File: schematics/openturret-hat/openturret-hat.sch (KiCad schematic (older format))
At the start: 6 parts, among them J1 Raspberry_Pi_2_3, U0 L293D, U1 L293D, U2 AMS1117-5.0, U3 AMS1117-5.0

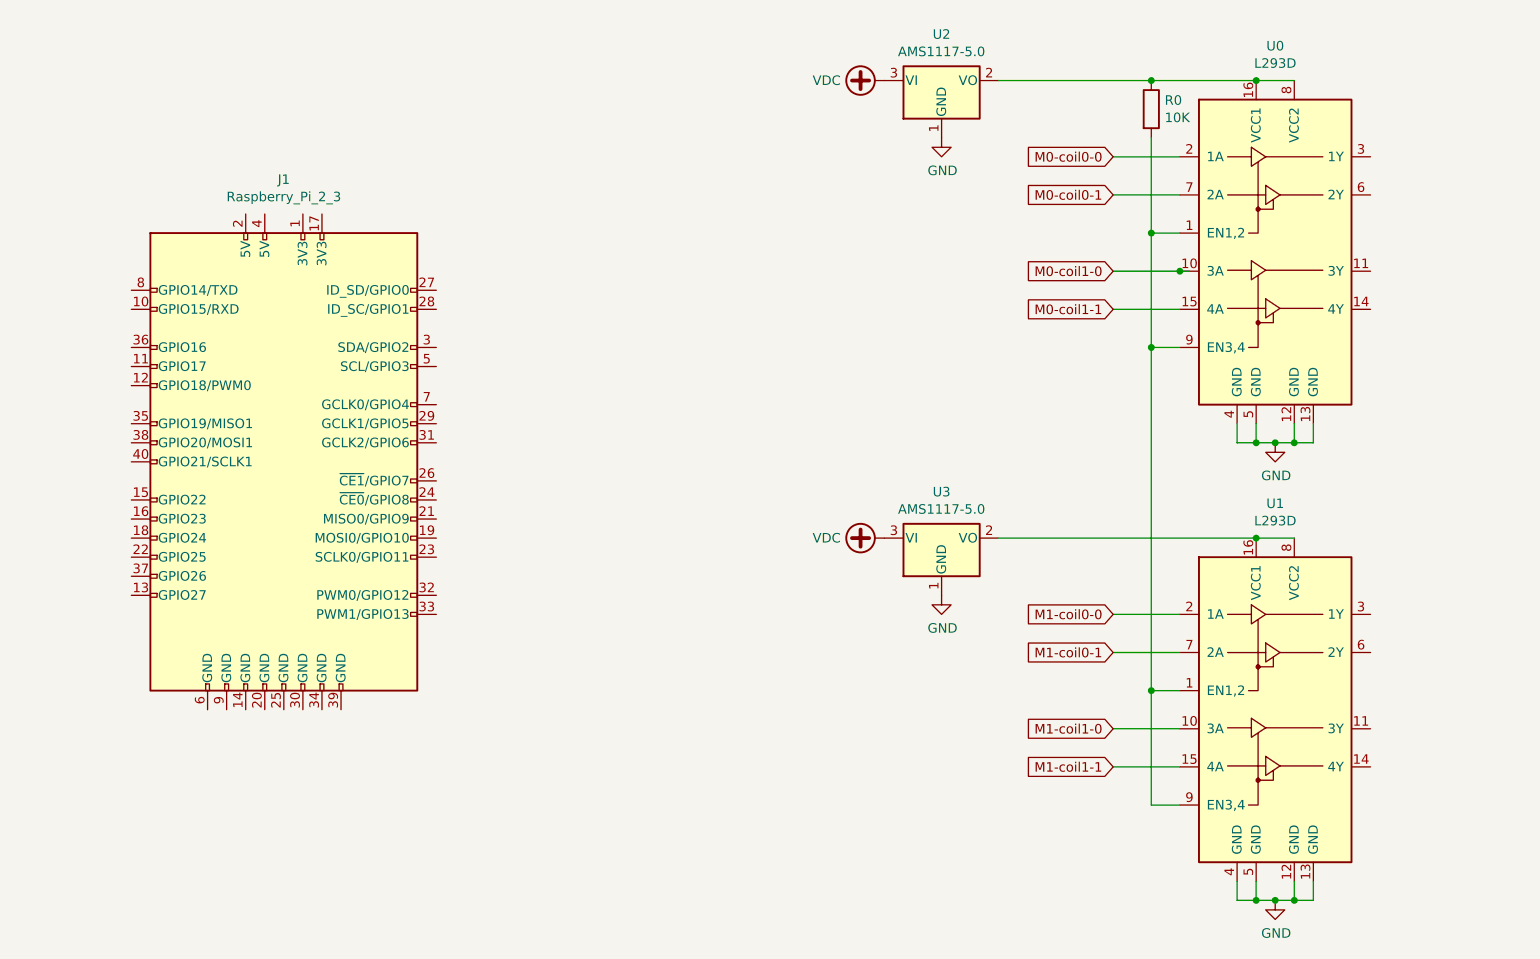
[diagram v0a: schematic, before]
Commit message: WIP on schematic and board layout
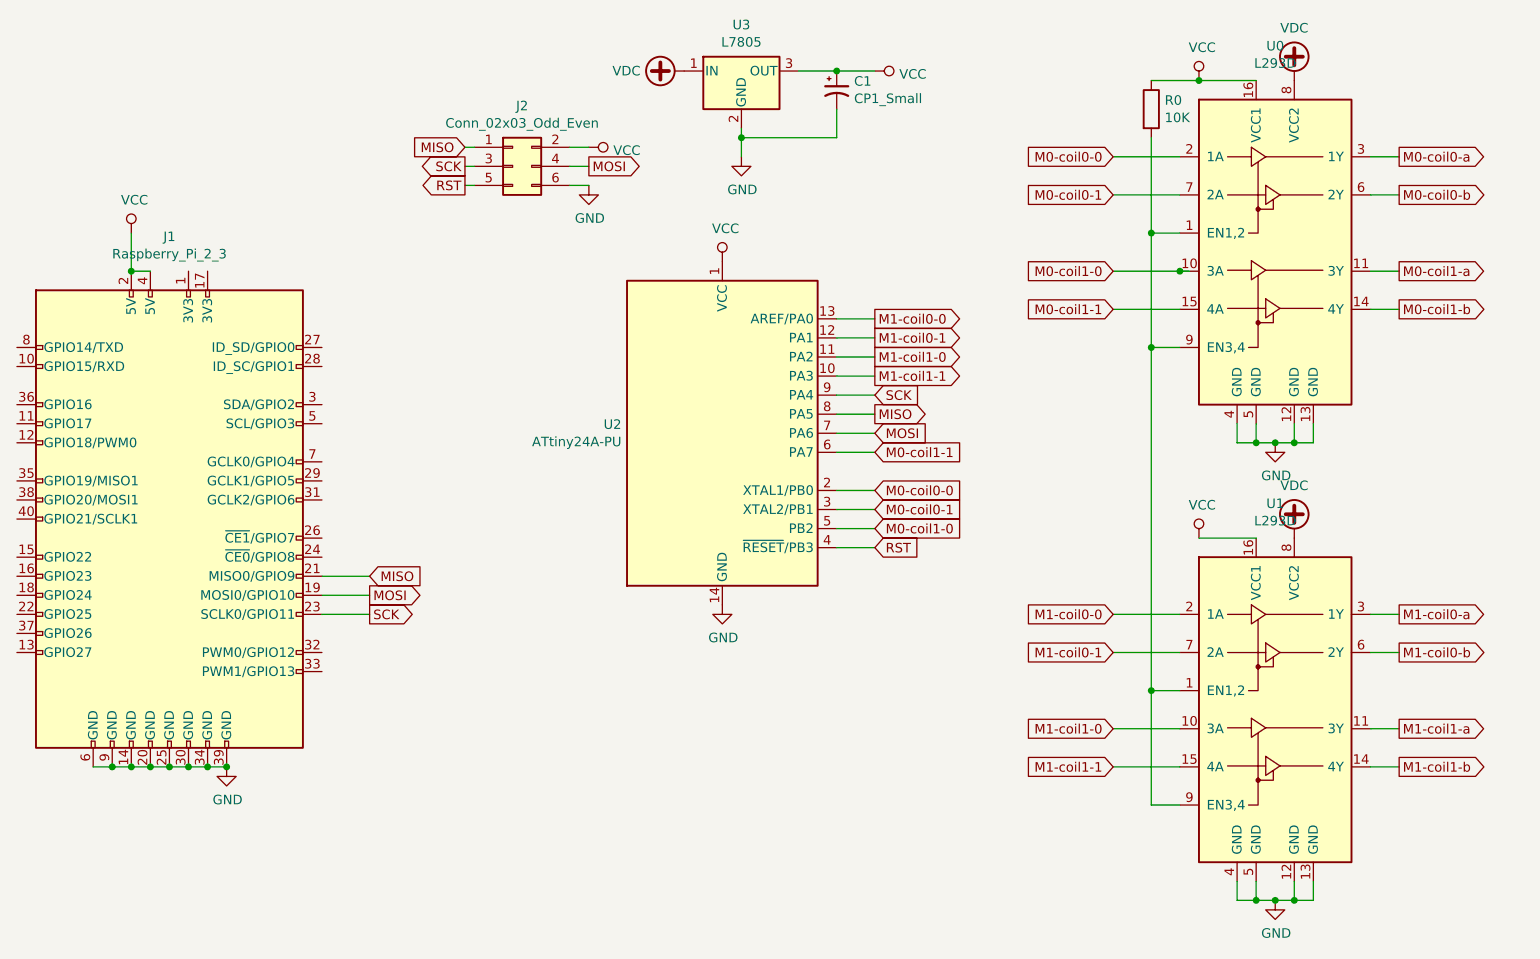
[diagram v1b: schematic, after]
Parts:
- removed U2, U3: AMS1117-5.0, Package_TO_SOT_SMD:SOT-223-3_TabPin2, symbol Regulator_Linear:AMS1117-5.0
- added C1: CP1_Small, Capacitor_THT:CP_Radial_D5.0mm_P2.50mm, symbol Device:CP1_Small
- added J2: Conn_02x03_Odd_Even, Connector_PinHeader_2.54mm:PinHeader_2x03_P2.54mm_Vertical, symbol Connector_Generic:Conn_02x03_Odd_Even
- added U2: ATtiny24A-PU, Package_DIP:DIP-14_W7.62mm, symbol MCU_Microchip_ATtiny:ATtiny24A-PU
- added U3: L7805, Package_TO_SOT_THT:TO-220-3_Vertical, symbol Regulator_Linear:L7805
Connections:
- net GND: now also J1.14 (GND), J1.20 (GND), J1.25 (GND), J1.30 (GND), J1.34 (GND), J1.39 (GND), J1.6 (GND), J1.9 (GND), C1.2, J2.6 (Pin_6), U2.14 (GND), U3.2 (GND)
- net M0-coil0-0: now also U2.2 (XTAL1/PB0)
- net M0-coil0-1: now also U2.3 (XTAL2/PB1)
- net M0-coil1-0: now also U2.5 (PB2)
- net M0-coil1-1: now also U2.6 (PA7)
- net M1-coil0-0: now also U2.13 (AREF/PA0)
- net M1-coil0-1: now also U2.12 (PA1)
- net M1-coil1-0: now also U2.11 (PA2)
- net M1-coil1-1: now also U2.10 (PA3)
- net VDC: now also U0.8 (VCC2), U1.8 (VCC2), U3.1 (IN)
- net M0-coil1-a: now reaches U0.11 (3Y)
- net M0-coil1-b: now reaches U0.14 (4Y)
- net VCC: now reaches R0.1, U0.16 (VCC1)
- net VCC: now also J1.2 (5V), J1.4 (5V), U1.16 (VCC1), C1.1, J2.2 (Pin_2), U2.1 (VCC), U3.3 (OUT); no longer U0.8 (VCC2)
- net M0-coil0-a: now reaches U0.3 (1Y)
- net M0-coil0-b: now reaches U0.6 (2Y)
- net M1-coil1-a: now reaches U1.11 (3Y)
- net M1-coil1-b: now reaches U1.14 (4Y)
- net M1-coil0-a: now reaches U1.3 (1Y)
- net M1-coil0-b: now reaches U1.6 (2Y)
- net MOSI: now reaches J1.19 (MOSI0/GPIO10)
- net MOSI: now also J2.4 (Pin_4), U2.7 (PA6)
- net MISO: now reaches J1.21 (MISO0/GPIO9)
- net MISO: now also J2.1 (Pin_1), U2.8 (PA5)
- net SCK: now reaches J1.23 (SCLK0/GPIO11)
- net SCK: now also J2.3 (Pin_3), U2.9 (PA4)
- new net RST: J2.5 (Pin_5), U2.4 (~RESET~/PB3)
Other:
- moved on the sheet: J1
